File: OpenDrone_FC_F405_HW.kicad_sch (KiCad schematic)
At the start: 89 parts, among them J1 Conn_01x05, J11 Conn_01x05, J12 Conn_01x05, J13 Conn_01x02, J14 Conn_01x02, J16 Conn_01x05, J17 Conn_02x03_Odd_Even, J2 Conn_01x02, J3 Conn_01x02, J4 Conn_01x02, J5 Conn_01x02, J6 Conn_01x08, J7 Conn_01x02, J8 Conn_01x04, J9 Conn_01x02, U1 STM32F405RGTx, U2 TPS54331, U4 MPU6000, U5 HMC5883L, U6 BMP280, U7 TPS54331, U8 Board, Y2 8Mhz

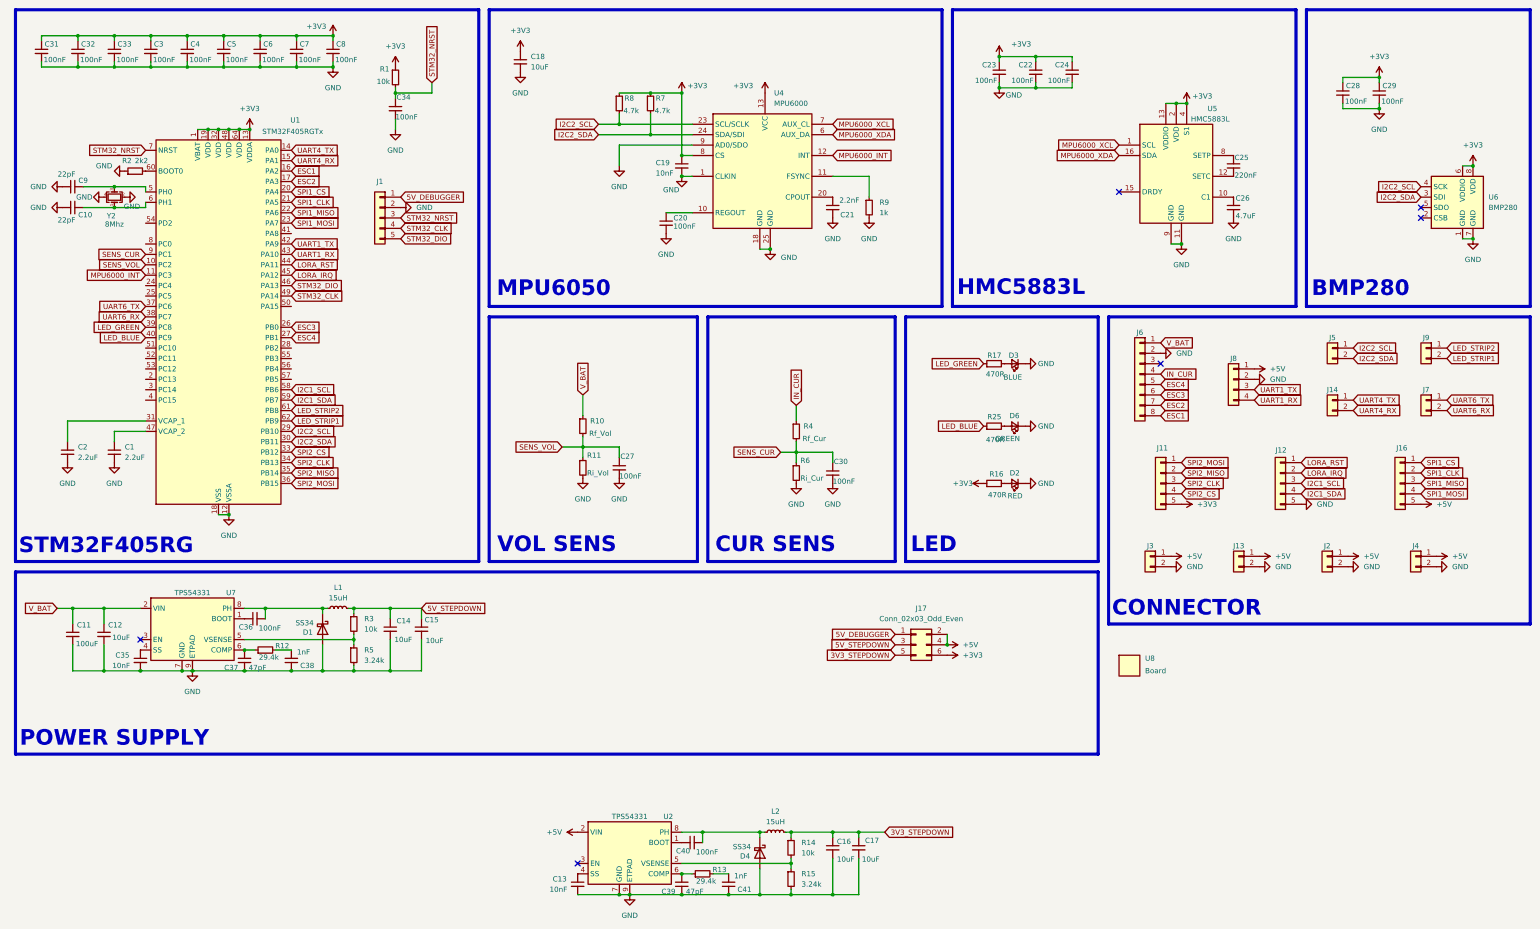
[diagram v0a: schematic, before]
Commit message: complete schematic & PCB v2.0
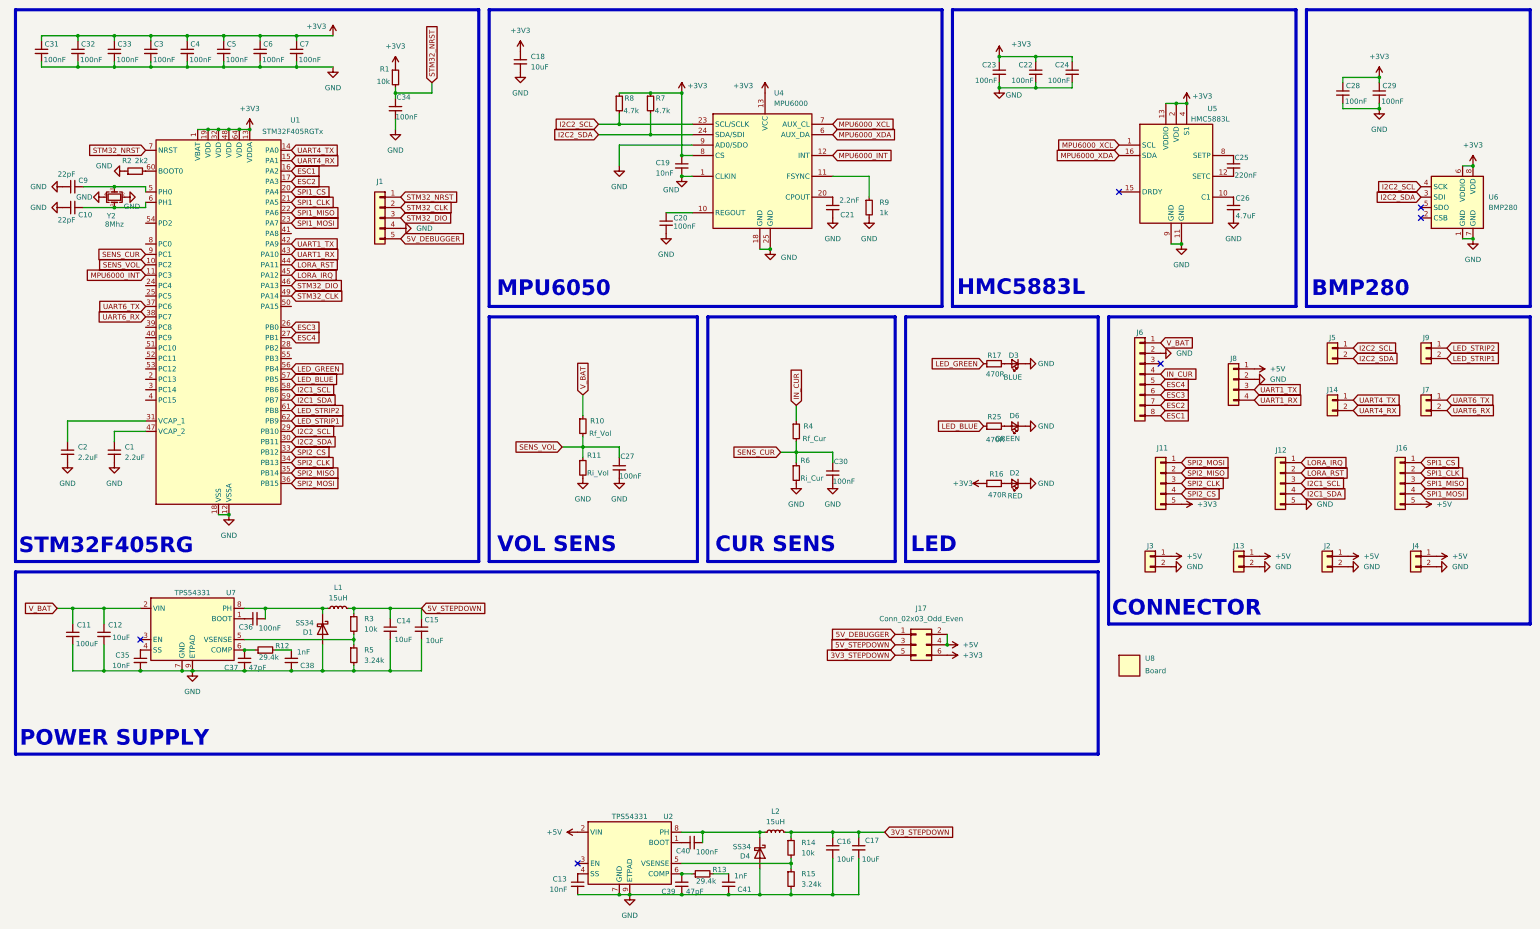
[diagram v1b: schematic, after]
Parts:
- removed C8: 100nF, Capacitor_SMD:C_0402_1005Metric, symbol Device:C_Small
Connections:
- net 5V_DEBUGGER: now also J1.5 (Pin_5); no longer J1.1 (Pin_1)
- net GND: now also J1.4 (Pin_4); no longer J1.2 (Pin_2)
- net LED_BLUE: now also U1.57 (PB5); no longer U1.40 (PC9)
- net LED_GREEN: now also U1.56 (PB4); no longer U1.39 (PC8)
- net LORA_IRQ: now also J12.1 (Pin_1); no longer J12.2 (Pin_2)
- net LORA_RST: now also J12.2 (Pin_2); no longer J12.1 (Pin_1)
- net STM32_CLK: now also J1.2 (Pin_2); no longer J1.4 (Pin_4)
- net STM32_DIO: now also J1.3 (Pin_3); no longer J1.5 (Pin_5)
- net STM32_NRST: now also J1.1 (Pin_1); no longer J1.3 (Pin_3)
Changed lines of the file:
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@@
 	)
 	(junction
-		(at 91.44 27.94)
-		(diameter 0)
-		(color 0 0 0 0)
-	)
-	(junction
 		(at 369.57 69.85)
 		(diameter 0)
@@
 	)
 	(junction
-		(at 91.44 20.32)
-		(diameter 0)
-		(color 0 0 0 0)
-	)
-	(junction
 		(at 68.58 43.18)
 		(diameter 0)
@@
 	(wire
 		(pts
-			(xy 91.44 27.94) (xy 91.44 26.67)
-		)
-		(stroke
-			(width 0)
-			(type default)
-		)
-	)
-	(wire
-		(pts
 			(xy 68.58 43.18) (xy 71.12 43.18)
 		)
@@
 	(wire
 		(pts
-			(xy 91.44 21.59) (xy 91.44 20.32)
-		)
-		(stroke
-			(width 0)
-			(type default)
-		)
-	)
-	(wire
-		(pts
 			(xy 96.52 166.37) (xy 96.52 167.64)
 		)
@@
 	(global_label "STM32_DIO"
 		(shape input)
-		(at 107.95 69.85 0)
+		(at 107.95 64.77 0)
 		(fields_autoplaced yes)
 		(effects
@@
 		)
 		(property "Intersheetrefs" "${INTERSHEET_REFS}"
-			(at 121.1556 69.85 0)
+			(at 121.1556 64.77 0)
 			(effects
 				(font
@@
 	(global_label "STM32_CLK"
 		(shape input)
-		(at 107.95 67.31 0)
+		(at 107.95 62.23 0)
 		(fields_autoplaced yes)
 		(effects
@@
 		)
 		(property "Intersheetrefs" "${INTERSHEET_REFS}"
-			(at 121.5184 67.31 0)
+			(at 121.5184 62.23 0)
 			(effects
 				(font
@@
 	(global_label "LED_GREEN"
 		(shape input)
-		(at 45.72 91.44 180)
+		(at 81.28 101.6 0)
 		(fields_autoplaced yes)
 		(effects
@@
 				(size 1.27 1.27)
 			)
-			(justify right)
+			(justify left)
 		)
 		(property "Intersheetrefs" "${INTERSHEET_REFS}"
-			(at 32.1516 91.44 0)
+			(at 94.8484 101.6 0)
 			(effects
 				(font
 					(size 1.27 1.27)
 				)
-				(justify right)
+				(justify left)
 				(hide yes)
 			)
@@
 	(global_label "LORA_RST"
 		(shape input)
-		(at 327.66 124.46 0)
+		(at 327.66 127 0)
 		(fields_autoplaced yes)
 		(effects
@@
 		)
 		(property "Intersheetrefs" "${INTERSHEET_REFS}"
-			(at 339.7771 124.46 0)
+			(at 339.7771 127 0)
 			(effects
 				(font
@@
 	(global_label "5V_DEBUGGER"
 		(shape input)
-		(at 107.95 59.69 0)
+		(at 107.95 69.85 0)
 		(fields_autoplaced yes)
 		(effects
@@
 		)
 		(property "Intersheetrefs" "${INTERSHEET_REFS}"
-			(at 124.1794 59.69 0)
+			(at 124.1794 69.85 0)
 			(effects
 				(font
@@
 	(global_label "STM32_NRST"
 		(shape input)
-		(at 107.95 64.77 0)
+		(at 107.95 59.69 0)
 		(fields_autoplaced yes)
 		(effects
@@
 		)
 		(property "Intersheetrefs" "${INTERSHEET_REFS}"
-			(at 122.7279 64.77 0)
+			(at 122.7279 59.69 0)
 			(effects
 				(font
@@
 	(global_label "LED_BLUE"
 		(shape input)
-		(at 45.72 93.98 180)
+		(at 81.28 104.14 0)
 		(fields_autoplaced yes)
 		(effects
@@
 				(size 1.27 1.27)
 			)
-			(justify right)
+			(justify left)
 		)
 		(property "Intersheetrefs" "${INTERSHEET_REFS}"
-			(at 33.5425 93.98 0)
+			(at 93.4575 104.14 0)
 			(effects
 				(font
 					(size 1.27 1.27)
 				)
-				(justify right)
+				(justify left)
 				(hide yes)
 			)
@@
 	(global_label "LORA_IRQ"
 		(shape input)
-		(at 327.66 127 0)
+		(at 327.66 124.46 0)
 		(fields_autoplaced yes)
 		(effects
@@
 		)
 		(property "Intersheetrefs" "${INTERSHEET_REFS}"
-			(at 339.5353 127 0)
+			(at 339.5353 124.46 0)
 			(effects
 				(font
@@
 	(symbol
 		(lib_id "power:GND")
-		(at 107.95 62.23 90)
+		(at 107.95 67.31 90)
 		(unit 1)
 		(exclude_from_sim no)
@@
 		(fields_autoplaced yes)
 		(property "Reference" "#PWR08"
-			(at 114.3 62.23 0)
+			(at 114.3 67.31 0)
 			(effects
 				(font
@@
 		)
 		(property "Value" "GND"
-			(at 111.76 62.2299 90)
+			(at 111.76 67.3099 90)
 			(effects
 				(font
@@
 		)
 		(property "Footprint" ""
-			(at 107.95 62.23 0)
+			(at 107.95 67.31 0)
 			(effects
 				(font
@@
 		)
 		(property "Datasheet" ""
-			(at 107.95 62.23 0)
+			(at 107.95 67.31 0)
 			(effects
 				(font
@@
 		)
 		(property "Description" "Power symbol creates a global label with name \"GND\" , ground"
-			(at 107.95 62.23 0)
+			(at 107.95 67.31 0)
 			(effects
 				(font
@@
 					(unit 1)
 				)
-			)
-		)
-	)
-	(symbol
-		(lib_id "Device:C_Small")
-		(at 91.44 24.13 0)
-		(unit 1)
-		(exclude_from_sim no)
-		(in_bom yes)
-		(on_board yes)
-		(dnp no)
-		(property "Reference" "C8"
-			(at 92.202 22.352 0)
-			(effects
-				(font
-					(size 1.27 1.27)
-				)
-				(justify left)
-			)
-		)
-		(property "Value" "100nF"
-			(at 91.948 26.162 0)
-			(effects
-				(font
-					(size 1.27 1.27)
-				)
-				(justify left)
-			)
-		)
-		(property "Footprint" "Capacitor_SMD:C_0402_1005Metric"
-			(at 91.44 24.13 0)
-			(effects
-				(font
-					(size 1.27 1.27)
-				)
-				(hide yes)
-			)
-		)
-		(property "Datasheet" "~"
-			(at 91.44 24.13 0)
-			(effects
-				(font
-					(size 1.27 1.27)
-				)
-				(hide yes)
-			)
-		)
-		(property "Description" "Unpolarized capacitor, small symbol"
-			(at 91.44 24.13 0)
-			(effects
-				(font
-					(size 1.27 1.27)
-				)
-				(hide yes)
-			)
-		)
-		(property "Availability" ""
-			(at 91.44 24.13 0)
-			(effects
-				(font
-					(size 1.27 1.27)
-				)
-				(hide yes)
-			)
-		)
-		(property "Check_prices" ""
-			(at 91.44 24.13 0)
-			(effects
-				(font
-					(size 1.27 1.27)
-				)
-				(hide yes)
-			)
-		)
-		(property "MANUFACTURER" ""
-			(at 91.44 24.13 0)
-			(effects
-				(font
-					(size 1.27 1.27)
-				)
-				(hide yes)
-			)
-		)
-		(property "MAXIMUM_PACKAGE_HEIGHT" ""
-			(at 91.44 24.13 0)
-			(effects
-				(font
-					(size 1.27 1.27)
-				)
-				(hide yes)
-			)
-		)
-		(property "MF" ""
-			(at 91.44 24.13 0)
-			(effects
-				(font
-					(size 1.27 1.27)
-				)
-				(hide yes)
-			)
-		)
-		(property "MP" ""
-			(at 91.44 24.13 0)
-			(effects
-				(font
-					(size 1.27 1.27)
-				)
-				(hide yes)
-			)
-		)
-		(property "PARTREV" ""
-			(at 91.44 24.13 0)
-			(effects
-				(font
-					(size 1.27 1.27)
-				)
-				(hide yes)
-			)
-		)
-		(property "Package" ""
-			(at 91.44 24.13 0)
-			(effects
-				(font
-					(size 1.27 1.27)
-				)
-				(hide yes)
-			)
-		)
-		(property "Price" ""
-			(at 91.44 24.13 0)
-			(effects
-				(font
-					(size 1.27 1.27)
-				)
-				(hide yes)
-			)
-		)
-		(property "Purchase-URL" ""
-			(at 91.44 24.13 0)
-			(effects
-				(font
-					(size 1.27 1.27)
-				)
-				(hide yes)
-			)
-		)
-		(property "STANDARD" ""
-			(at 91.44 24.13 0)
-			(effects
-				(font
-					(size 1.27 1.27)
-				)
-				(hide yes)
-			)
-		)
-		(property "SnapEDA_Link" ""
-			(at 91.44 24.13 0)
-			(effects
-				(font
-					(size 1.27 1.27)
-				)
-				(hide yes)
-			)
-		)
-		(pin "1"
-		)
-		(pin "2"
-		)
-		(instances
-			(project "OpenDrone_FC_F405_HW"
-				(path "/164a3579-a590-4494-9ab2-e38048782624"
-					(reference "C8")
-					(unit 1)
-				)
